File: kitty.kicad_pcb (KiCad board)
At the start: 2 copper layers, 50.4 x 41.7 mm, 2 parts

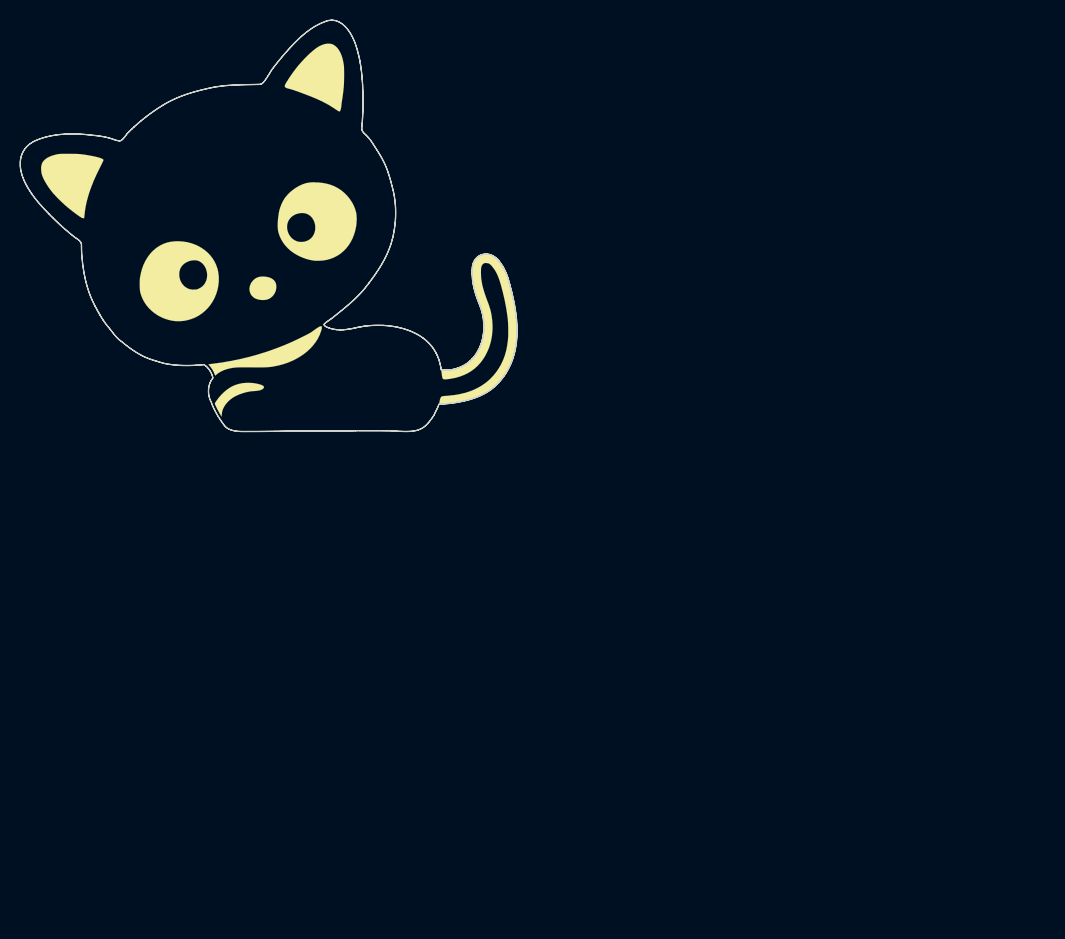
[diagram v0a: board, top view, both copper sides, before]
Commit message: finish layout
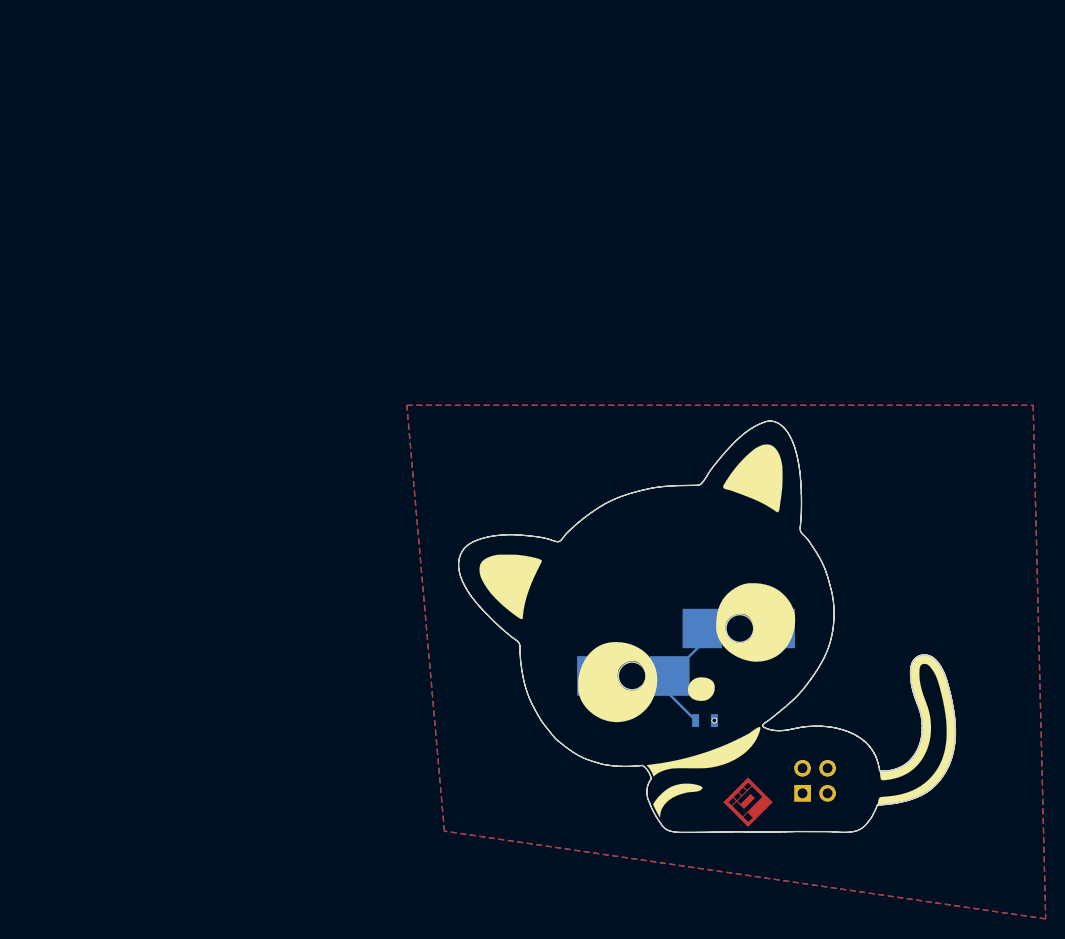
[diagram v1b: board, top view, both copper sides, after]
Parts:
- removed the G*** at (0.00, 0.00) (x2)
- added ?: , kitty:p_logo_5_copper, F.Cu at (48.6, 54.2)
- added D1: LED, kitty:LED, B.Cu at (45.3, 36.6)
- added D2: LED, kitty:LED, B.Cu at (39.2, 41.4)
- added G*** (x2): LOGO, LOGO, F.Cu at (44.5, 40.6)
- added R1: 220R, Resistors_SMD:R_0805, B.Cu at (44.2, 45.9)
- added SAO1: 2x2, Pin_Headers:Pin_Header_Straight_2x02_Pitch2.54mm, B.Cu at (54.1, 53.3)
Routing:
- net Net-(D1-Pad1): track 0.00 -> 11.8 mm
- net GND: vias 0 -> 1
- added copper zone on B.Cu, net +3V3
- added copper zone on F.Cu, net GND
